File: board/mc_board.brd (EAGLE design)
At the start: 41.1 x 26.4 mm, 16 parts, among them IC1 MEGA8-P, Q1 16MHz

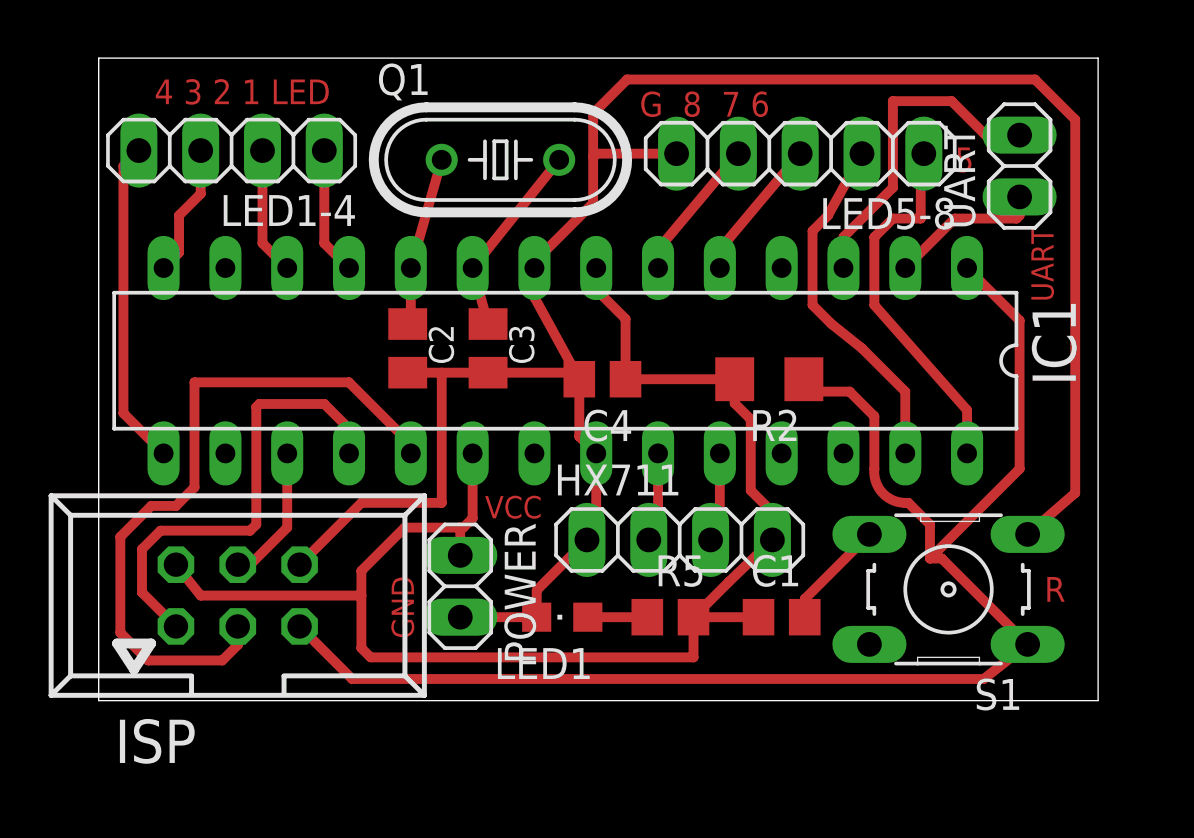
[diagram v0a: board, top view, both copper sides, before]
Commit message: improved board layout
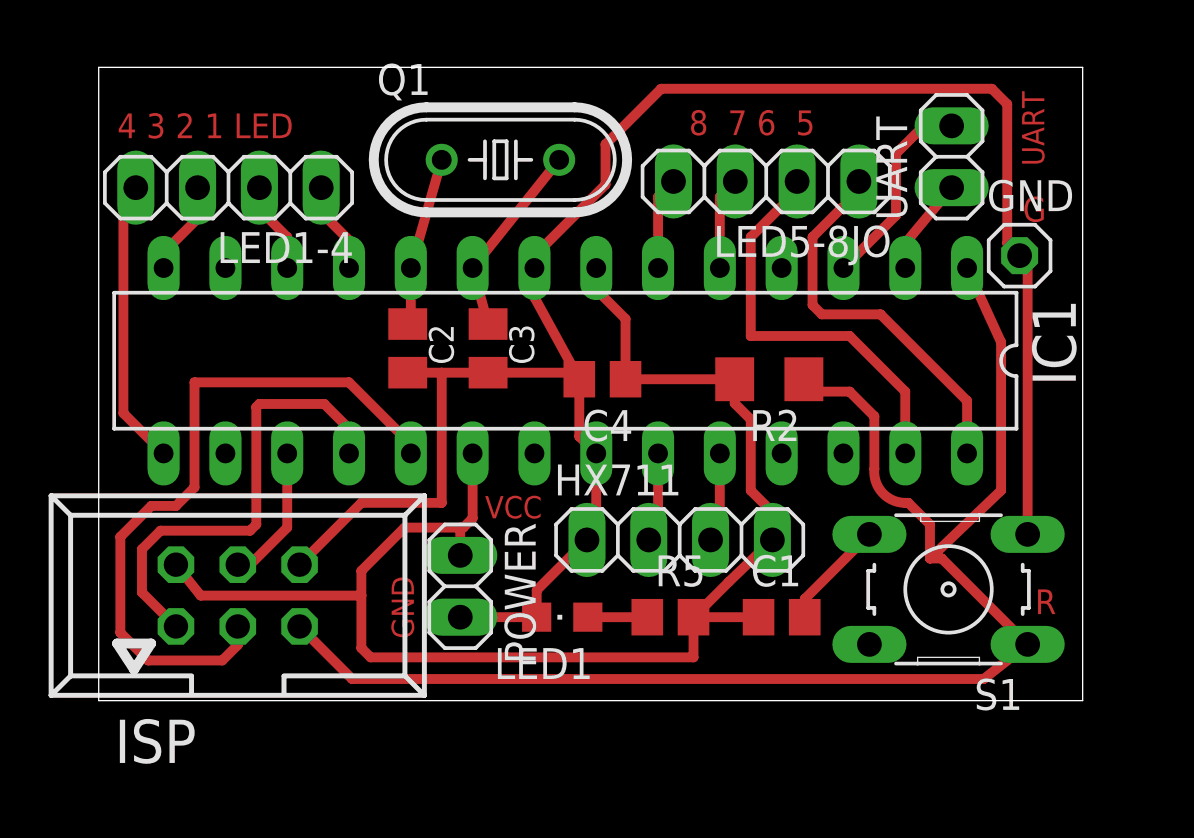
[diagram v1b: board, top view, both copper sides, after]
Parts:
- removed LED5-8: JP2, pinhead:1X05
- added GND: Gnd, pinhead:1X01
- added LED5-8JO: JP2, pinhead:1X04
- moved UART 2.82 mm to (35.1, 22.4)
- moved LED1-4 1.53 mm to (5.33, 21.1)
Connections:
- net GND: now also GND.1; no longer LED5-8.5
- net PC4/LED6: now also LED5-8JO.2; no longer LED5-8.2
- net PC5/LED5: now also LED5-8JO.1; no longer LED5-8.1
- net PD3/LED7: now also LED5-8JO.3; no longer LED5-8.3
- net PD4/LED8: now also LED5-8JO.4; no longer LED5-8.4
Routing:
- net GND: track 88.5 -> 80.7 mm
- net PD1/UART: track 13.5 -> 8.35 mm
- net PC4/LED6: track 14.6 -> 17.0 mm
- net PD0/UART: track 6.36 -> 3.99 mm
- net PD4/LED8: track 5.90 -> 3.82 mm
- net PD3/LED7: track 5.90 -> 3.82 mm
- net PB0/LED3: track 5.46 -> 3.88 mm
- net PB1/LED4: track 13.4 -> 11.8 mm
- net PD6/LED2: track 5.25 -> 3.78 mm
- net PD5/LED1: track 5.25 -> 3.78 mm
- net RESET: track 61.5 -> 60.6 mm
- net PC5/LED5: track 15.3 -> 16.0 mm
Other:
- board size 41.1 x 26.4 mm -> 40.4 x 26 mm
- board text added: "8 7 6 5"
- board text added: "G"
- board text removed: "5"
- board text removed: "G 8 7 6"

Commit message: even better board layout
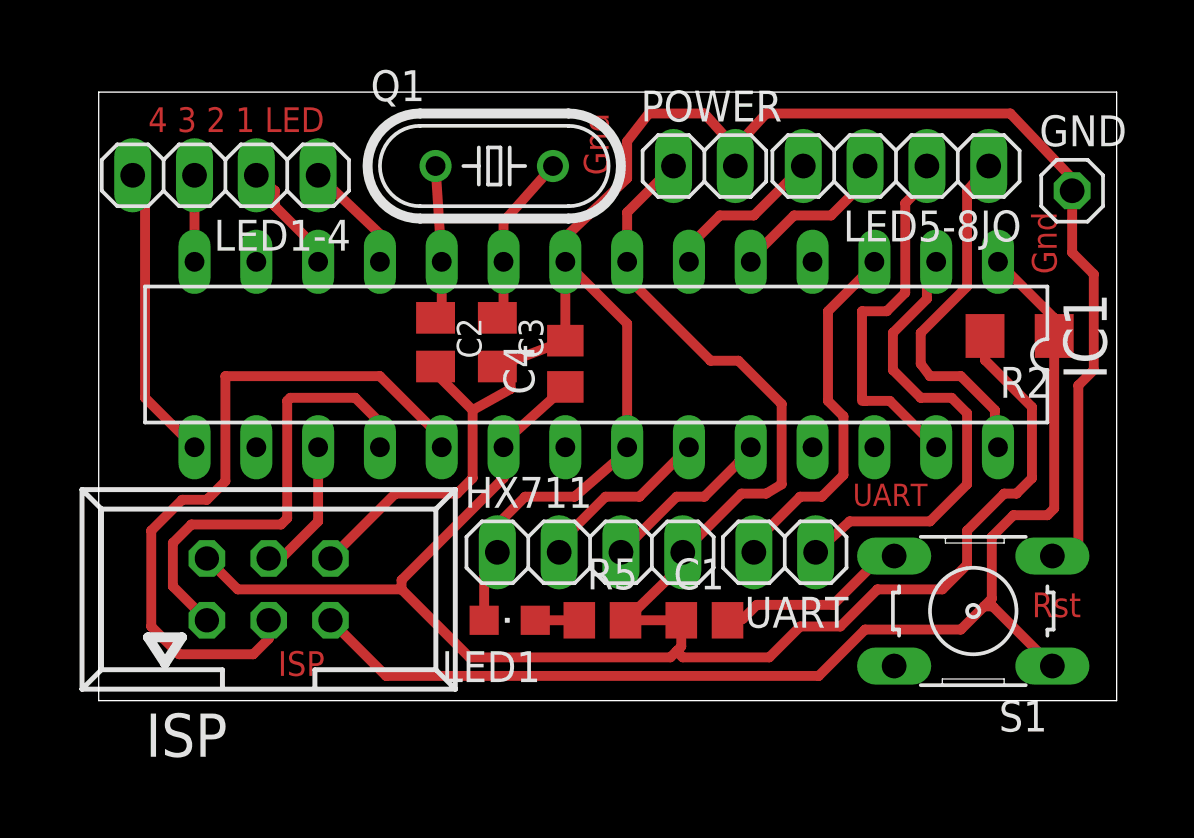
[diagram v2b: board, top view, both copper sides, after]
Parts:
- moved POWER 20.0 mm to (24.9, 22.0), turned to 0 degrees
- moved UART 17.6 mm to (28.2, 6.10), turned to 180 degrees
- moved R2 10.4 mm to (37.8, 15.0)
- moved LED5-8JO 5.37 mm to (32.8, 22.0)
- moved HX711 3.72 mm to (20.2, 6.10)
- moved GND 3.43 mm to (40.0, 21.0)
- moved C1 3.18 mm to (24.9, 3.30)
- moved R5 2.80 mm to (20.7, 3.30)
- moved LED1 2.16 mm to (16.9, 3.30)
- moved C4 1.65 mm to (19.2, 13.8), turned to 90 degrees
- moved S1 1.35 mm to (35.9, 3.68)
- moved ISP 1.30 mm to (6.99, 4.57)
- moved IC1 1.30 mm to (20.4, 14.2)
- moved C2 1.17 mm to (13.8, 14.7)
- moved LED1-4 0.52 mm to (5.21, 21.6)
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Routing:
- net +5V: track 60.2 -> 87.8 mm
- net PD0/UART: track 3.99 -> 19.2 mm
- net RESET: track 60.6 -> 49.9 mm
- net PD1/UART: track 8.35 -> 15.0 mm
- net GND: track 80.7 -> 86.9 mm
- net PC0/DT: track 3.71 -> 7.35 mm
- net PC1/SCK: track 3.71 -> 7.17 mm
- net N$9: track 4.50 -> 7.92 mm
- net PD3/LED7: track 3.82 -> 6.78 mm
- net PD4/LED8: track 3.82 -> 6.70 mm
- net PC4/LED6: track 17.0 -> 15.2 mm
- net PC5/LED5: track 16.0 -> 14.7 mm
- net N$6: track 7.43 -> 6.35 mm
- net N$5: track 8.08 -> 7.15 mm
- net PD6/LED2: track 3.78 -> 4.65 mm
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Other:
- board size 40.4 x 26 mm -> 41.8 x 25 mm
- board text added: "Gnd"
- board text added: "ISP"
- board text added: "Rst"
- board text removed: "8 7 6 5"
- board text removed: "G"
- board text removed: "GND"
- board text removed: "R"
- board text removed: "VCC"
